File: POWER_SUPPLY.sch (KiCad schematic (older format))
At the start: 15 parts, among them J10 Conn_02x12_Odd_Even, J11 X_LIMIT1, J12 Y_LIMIT1, J13 Z_LIMIT1, J14 PROBE, J15 START, J16 HOLD, J17 X_LIMIT2, J18 Y_LIMIT2, J19 Z_LIMIT2, J8 MOTOR

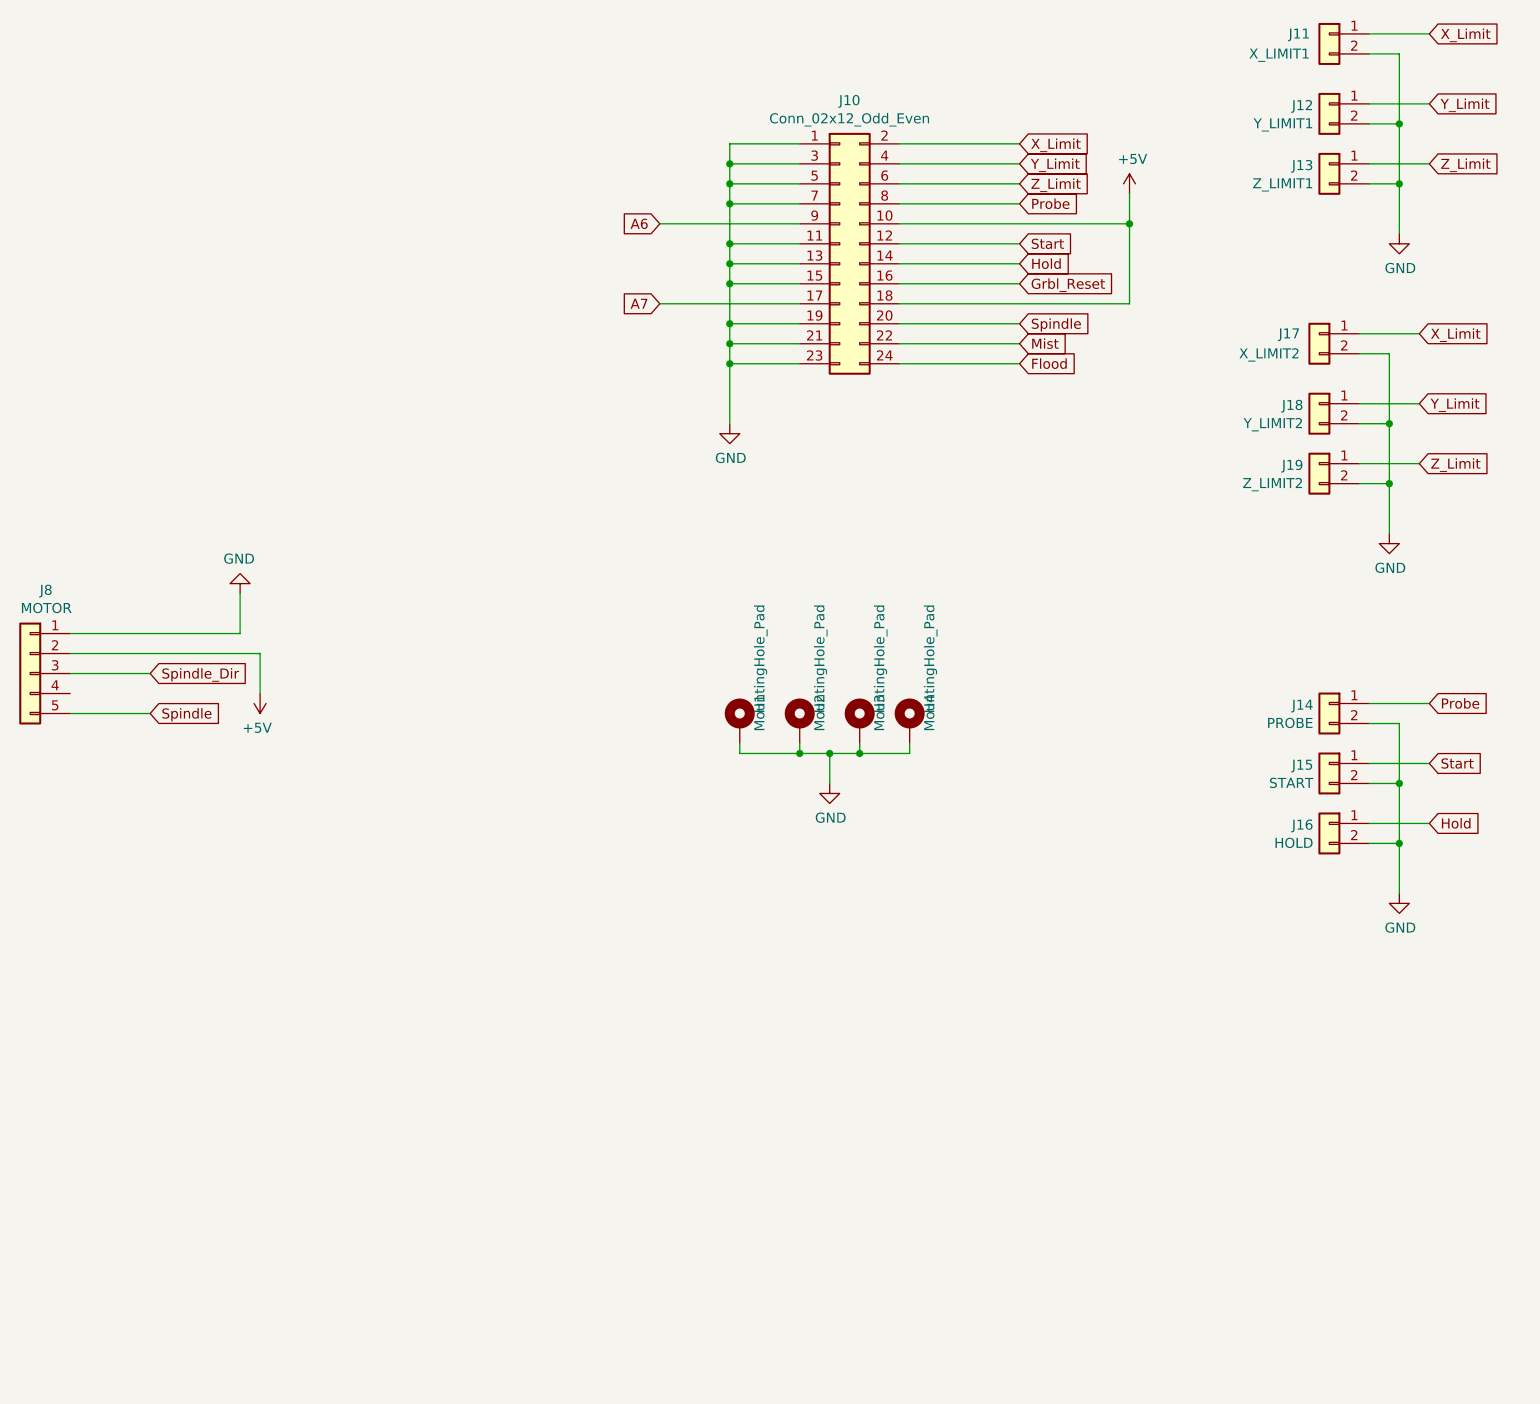
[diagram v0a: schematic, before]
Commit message: update,
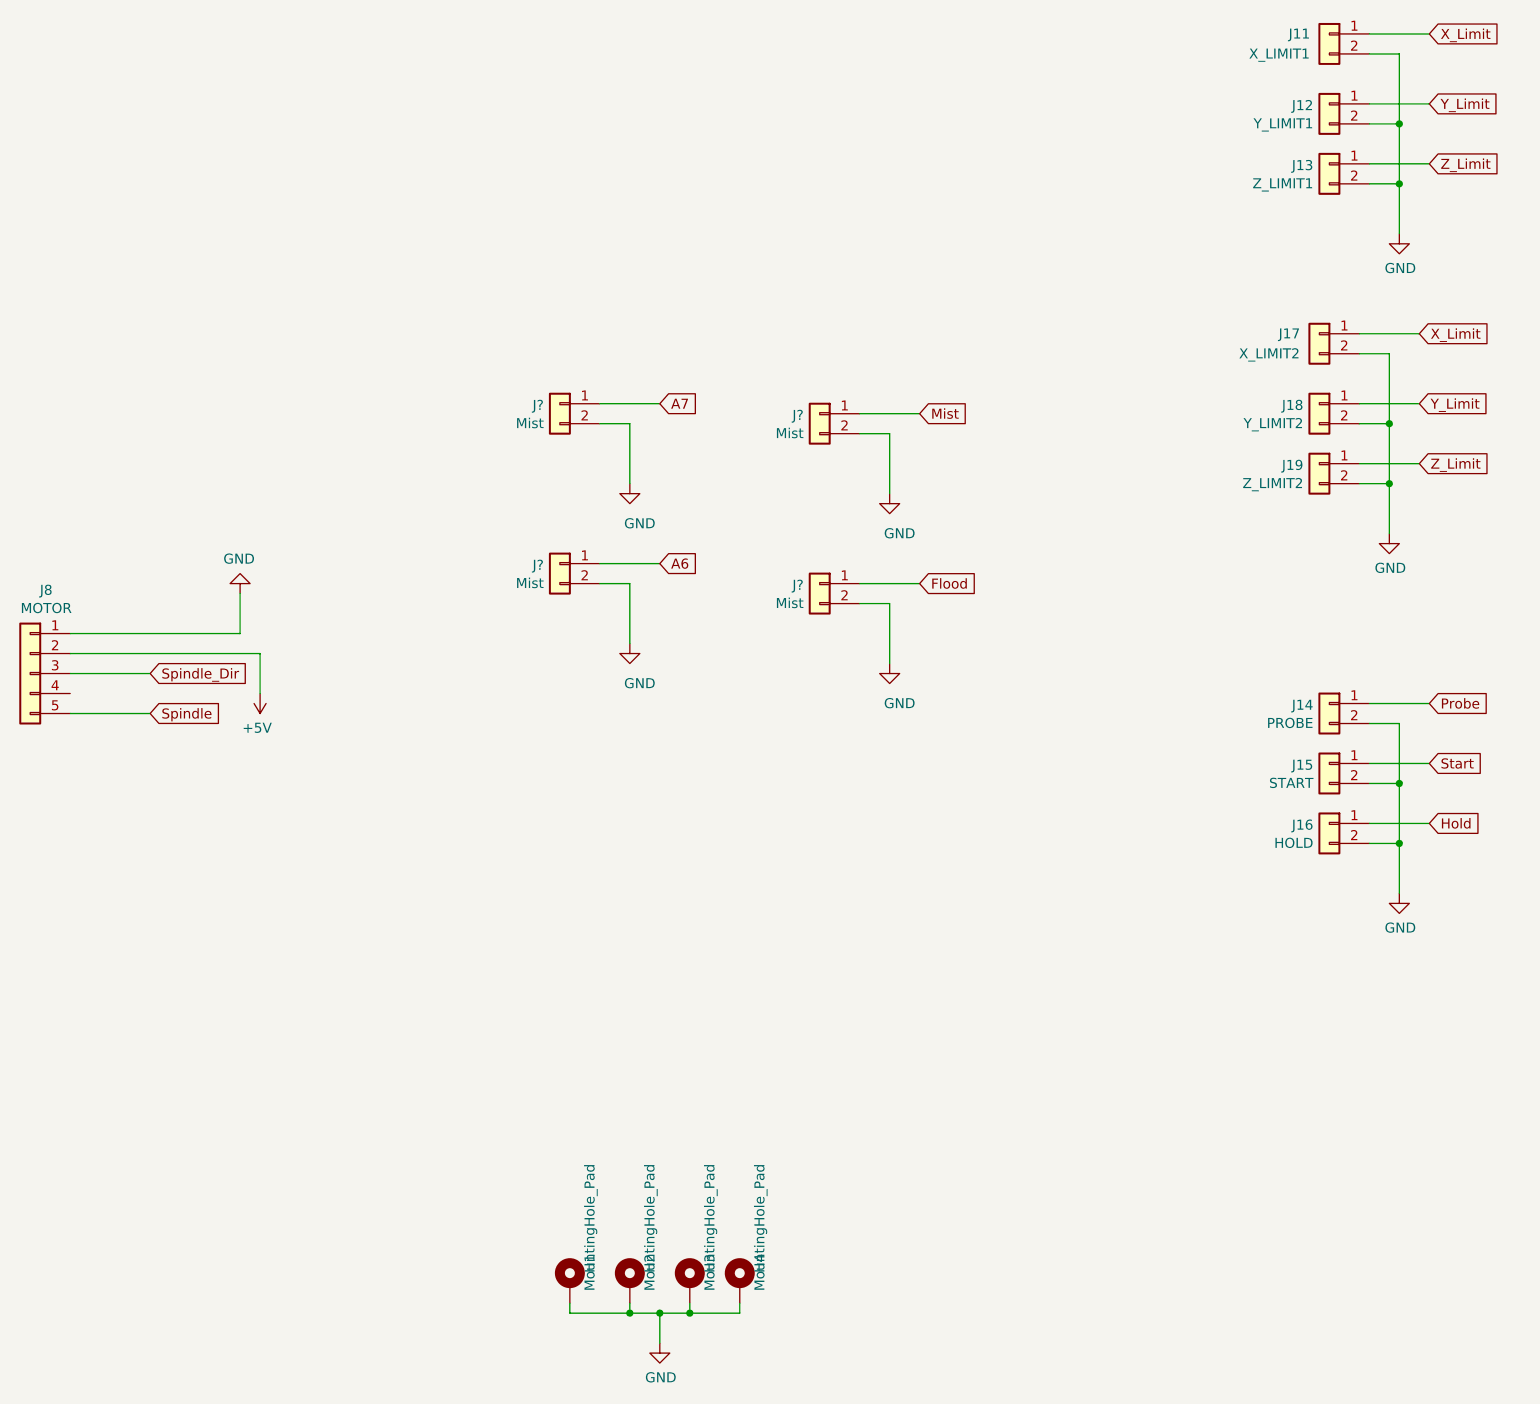
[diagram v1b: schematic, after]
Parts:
- removed J10: Conn_02x12_Odd_Even, Connector_PinHeader_2.54mm:PinHeader_2x12_P2.54mm_Vertical, symbol Connector_Generic:Conn_02x12_Odd_Even
- added J? (x4): Mist, Connector_JST:JST_XH_S02B-XH-A-1_1x02_P2.50mm_Horizontal, symbol Connector_Generic:Conn_01x02
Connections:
- net A6: now also J?.1 (Pin_1)
- net A7: now also J?.1 (Pin_1)
- net Flood: now also J?.1 (Pin_1)
- net GND: now also J?.2 (Pin_2), J?.2 (Pin_2), J?.2 (Pin_2), J?.2 (Pin_2)
- net Mist: now also J?.1 (Pin_1)
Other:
- moved on the sheet: H1, H2, H3, H4
